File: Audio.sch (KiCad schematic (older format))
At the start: 5 parts

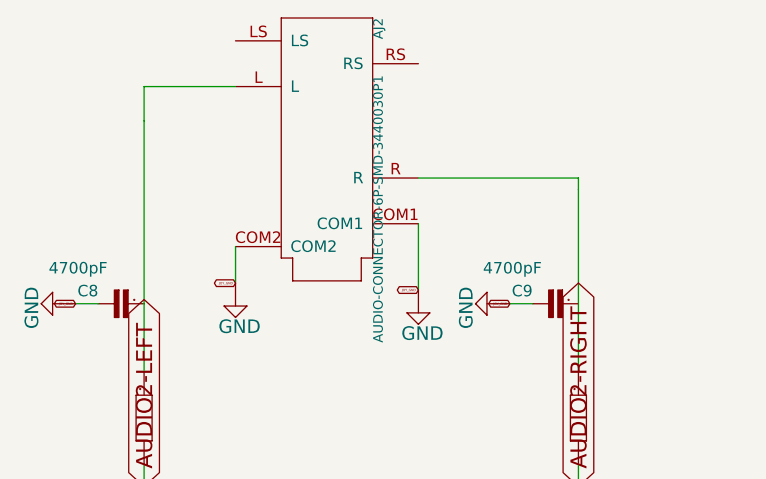
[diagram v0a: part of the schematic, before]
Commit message: Revision 2, needs extra check.
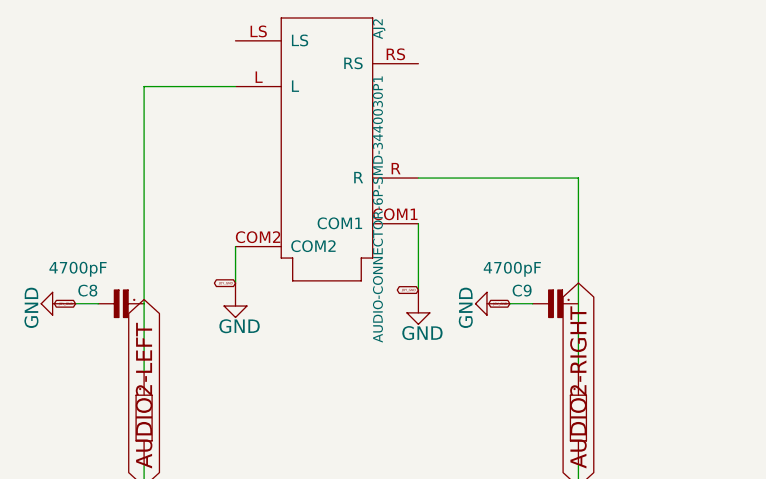
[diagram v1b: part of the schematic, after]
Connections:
- wire segments 14 -> 12
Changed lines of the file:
@@
 $Descr User 12505 8268
 encoding utf-8
-Sheet 1 8
+Sheet 5 8
 Title ""
 Date ""
@@
 	7200 2800 7200 2500
 Wire Wire Line
-	7200 2500 7200 1700
-Wire Wire Line
-	7200 1700 7200 1550
-Wire Wire Line
 	7200 1550 7600 1550
 Wire Wire Line
 	9100 2800 9100 2500
-Wire Wire Line
-	9100 2500 9100 2000
-Wire Wire Line
-	9100 2000 9100 1950
 Wire Wire Line
 	9100 1950 8400 1950
@@
 	1    0    0    -1
 $EndComp
+Wire Wire Line
+	7200 1550 7200 2500
+Wire Wire Line
+	9100 1950 9100 2500
 $EndSCHEMATC
